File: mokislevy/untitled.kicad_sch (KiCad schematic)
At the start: 2 parts, among them U1 STUSB4500QTR, U2 MAX17506ATP_T

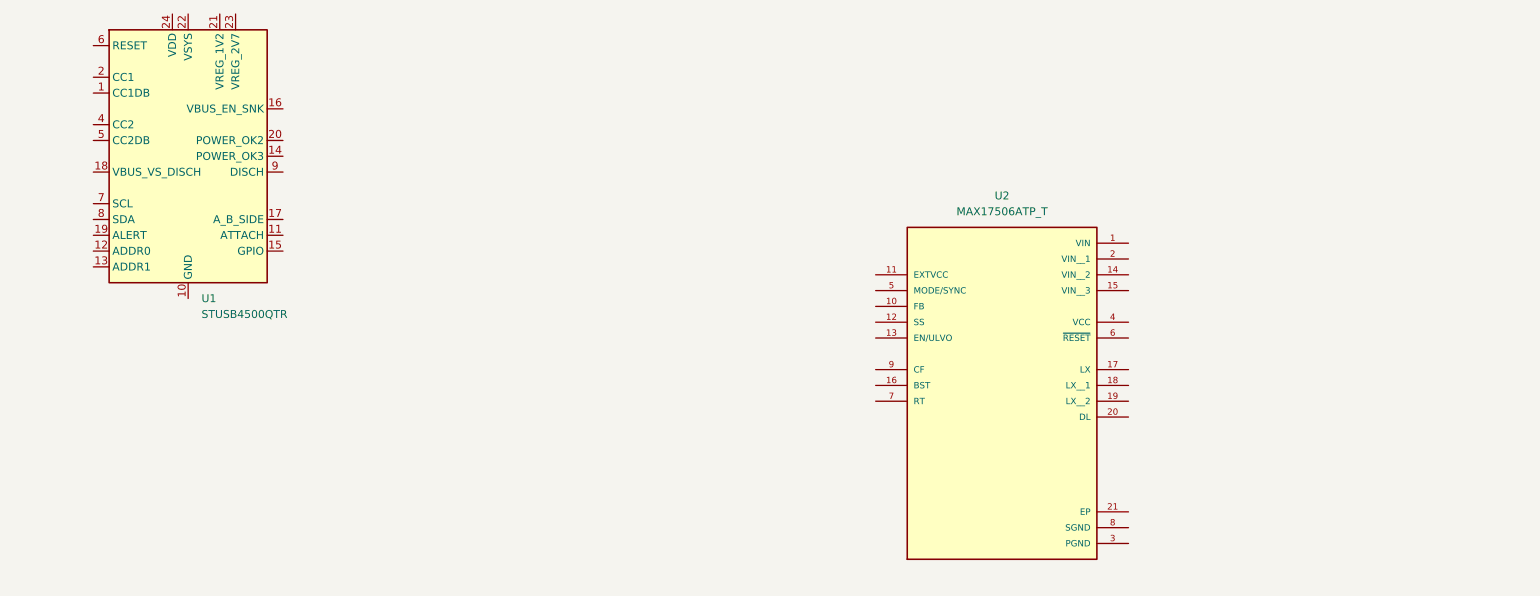
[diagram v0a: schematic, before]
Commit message: 28.7 päivitykset
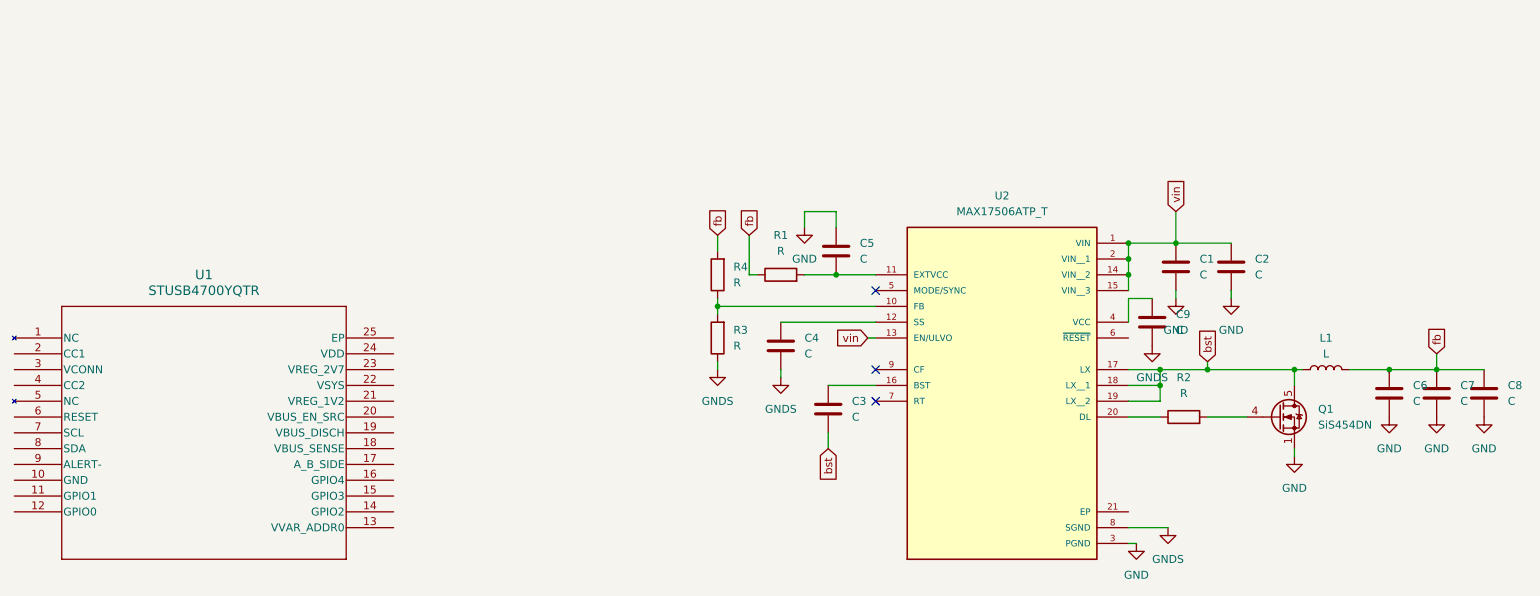
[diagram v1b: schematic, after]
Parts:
- removed U1: STUSB4500QTR, Package_DFN_QFN:QFN-24-1EP_4x4mm_P0.5mm_EP2.7x2.7mm, symbol Interface_USB:STUSB4500QTR
- added C1, C2, C3, C4, C5, C6, C7, C8, C9: C, symbol Device:C
- added L1: L, symbol Device:L
- added Q1: SiS454DN, Package_SO:Vishay_PowerPAK_1212-8_Single, symbol Transistor_FET:SiS454DN
- added R1, R2, R3, R4: R, symbol Device:R
- added U1: STUSB4700YQTR, QFN_700QTR_STM, symbol imported_components:STUSB4700YQTR
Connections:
- net vin: now reaches U2.1 (VIN)
- net vin: now also U2.13 (EN/ULVO), U2.14 (VIN__2), U2.15 (VIN__3), U2.2 (VIN__1), C1.1, C2.1
- net at U2.10 (FB): now also R3.2, R4.1
- net at U2.11 (EXTVCC): now also C5.2, R1.2
- net at U2.12 (SS): now also C4.1
- net at U2.16 (BST): now also C3.1
- net bst: now reaches U2.17 (LX)
- net bst: now also U2.18 (LX__1), U2.19 (LX__2), C3.2, L1.1, Q1.5 (D)
- net at U2.20 (DL): now also R2.1
- net GND: now reaches U2.3 (PGND)
- net GND: now also C1.2, C2.2, C5.1, C6.2, C7.2, C8.2, Q1.1 (S), Q1.2 (S), Q1.3 (S)
- net at U2.4 (VCC): now also C9.1
- net GNDS: now reaches U2.8 (SGND)
- net GNDS: now also C4.2, C9.2, R3.1
- new net: Q1.4 (G), R2.2
- new net fb: C6.1, C7.1, C8.1, L1.2, R1.1, R4.2
- no-connect marks 0 -> 3
